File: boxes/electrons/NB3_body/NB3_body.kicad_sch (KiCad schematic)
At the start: 47 parts, among them J1 Conn_02x05_Counter_Clockwise, J10 JST SH 4-way Socket, J11 JST SH 4-way Socket, J12 Conn_02x03_Top_Bottom, J13 Conn_02x03_Top_Bottom, J14 Conn_02x05_Counter_Clockwise, J15 Conn_02x05_Counter_Clockwise, J2 Conn_02x05_Counter_Clockwise, J3 Conn_02x05_Counter_Clockwise, J4 Conn_02x05_Counter_Clockwise, J5 Conn_02x05_Counter_Clockwise, J6 Conn_02x05_Counter_Clockwise, J7 Conn_02x07_Odd_Even, J8 Conn_02x07_Odd_Even, J9 Conn_02x07_Odd_Even

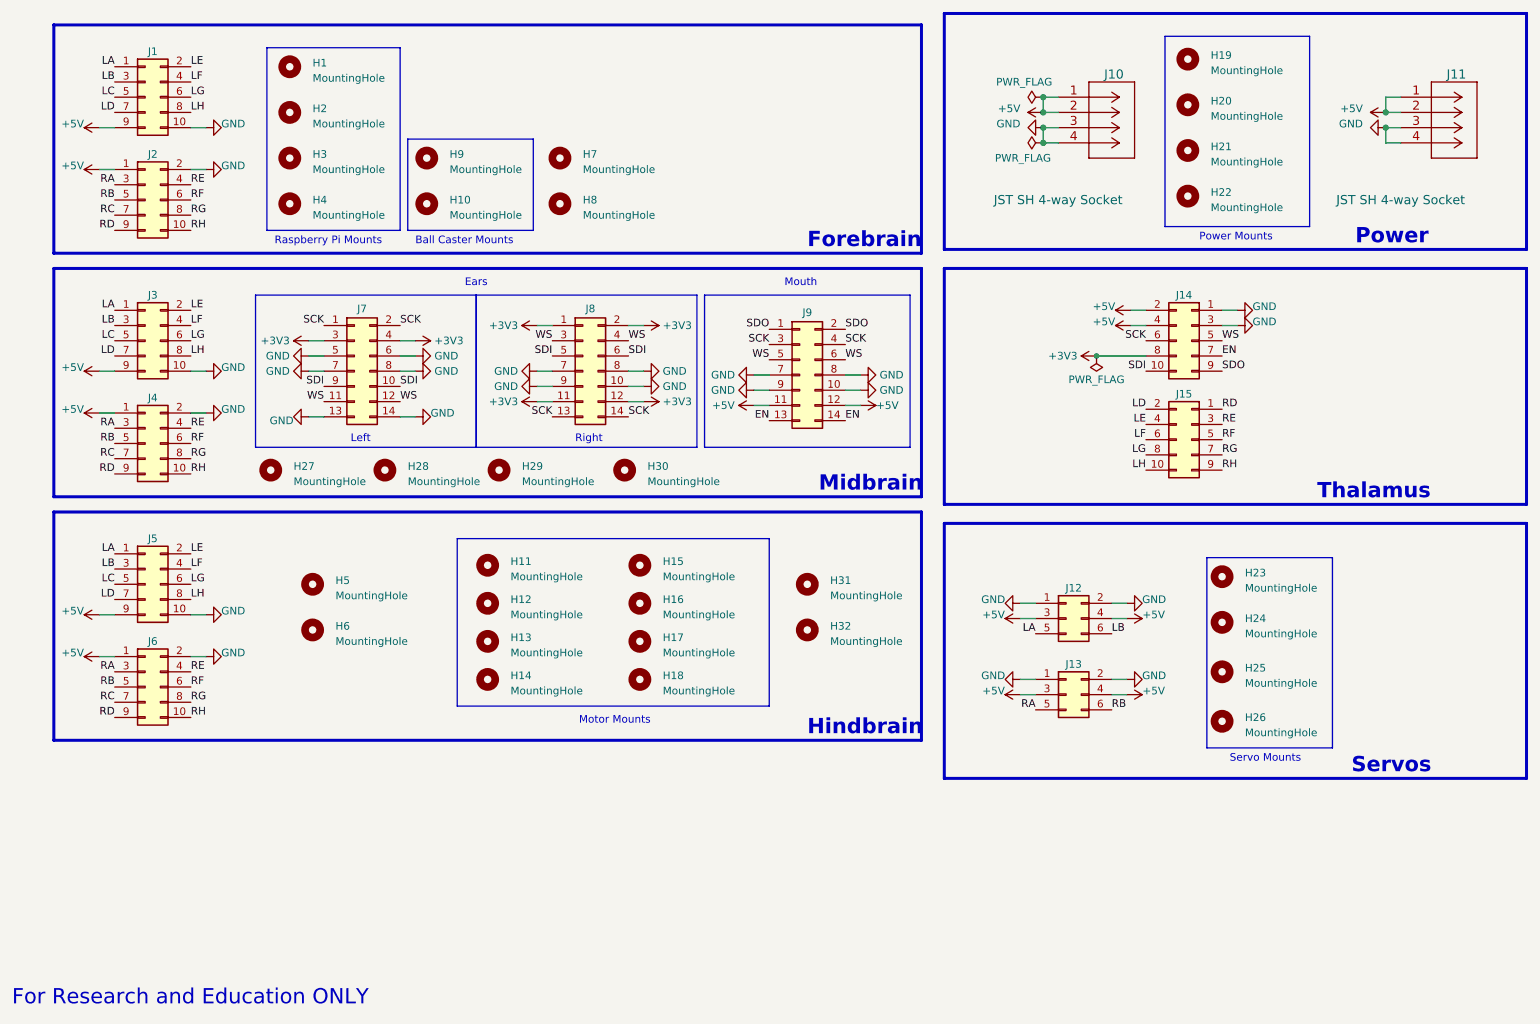
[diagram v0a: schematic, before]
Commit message: Update NB3 Body (rev 6)
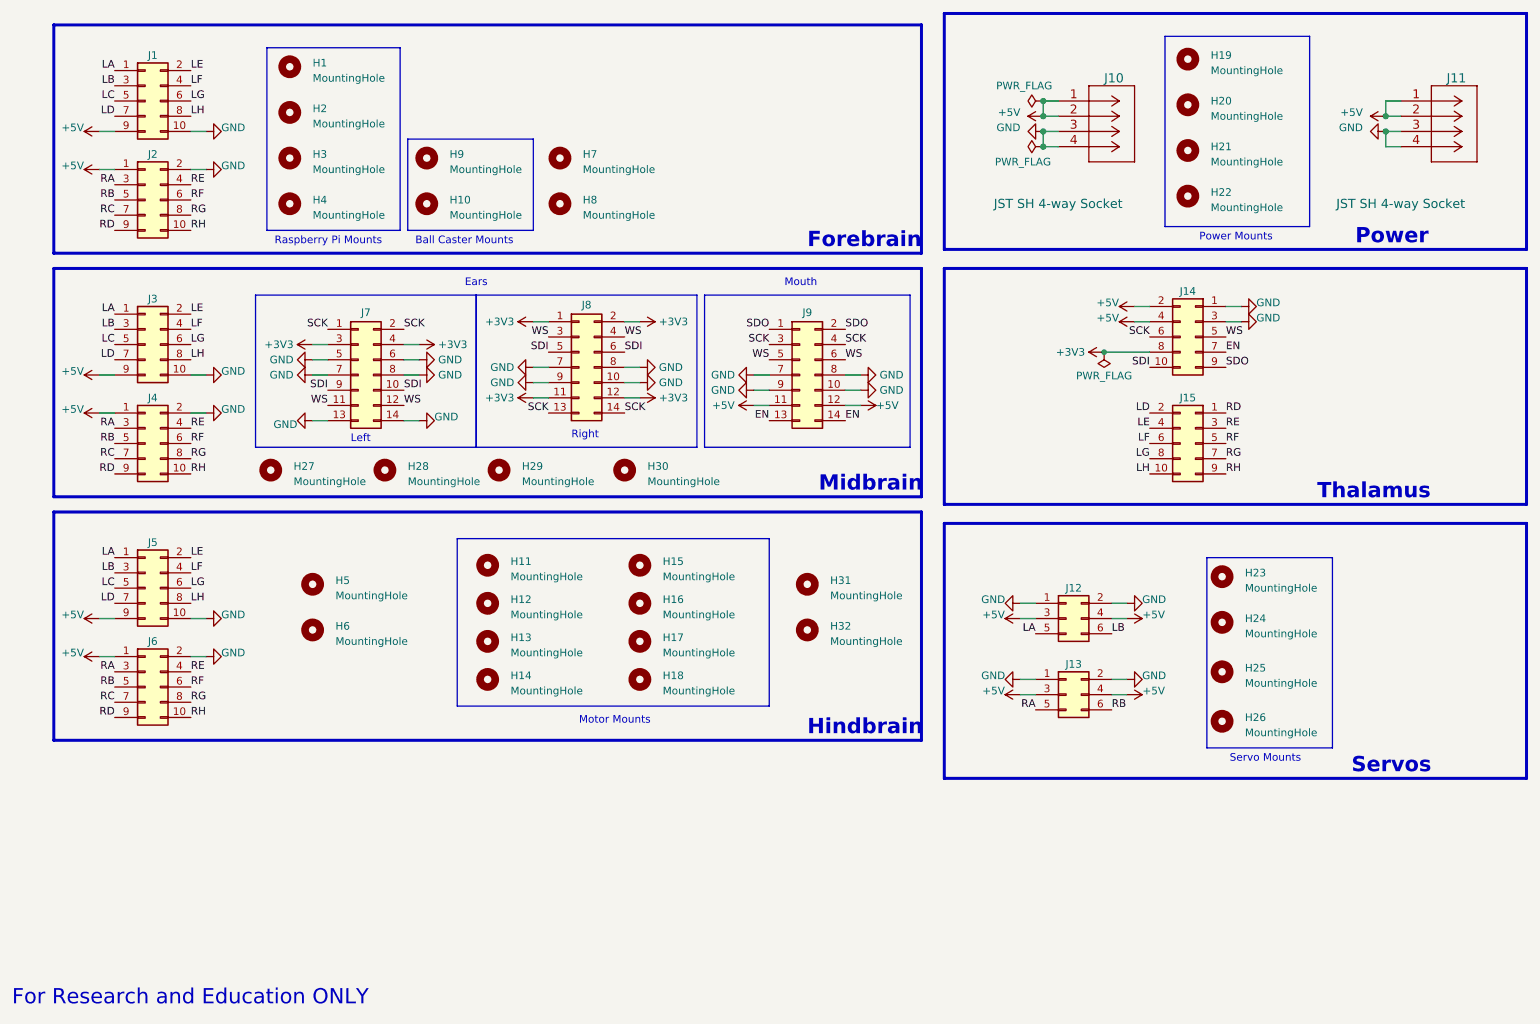
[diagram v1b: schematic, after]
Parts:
- J12, J13: footprint Connector_PinHeader_2.54mm:PinHeader_2x03_P2.54mm_Vertical_SMD -> Connector_PinHeader_2.54mm:PinHeader_2x03_P2.54mm_Vertical
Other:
- moved on the sheet: J1, J10, J11, J14, J15, J3, J5, J7, J8
